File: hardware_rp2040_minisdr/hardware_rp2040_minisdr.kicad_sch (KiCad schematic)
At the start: 0 parts

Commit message: started with schematic
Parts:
- added C1: C, symbol Device:C
- added C10, C11, C12, C13, C14, C15, C6, C7, C9: 100n, symbol Device:C
- added C16, C8: 1u, symbol Device:C
- added C2, C3: 15p, symbol Device:C
- added C4, C5: 10u, symbol Device:C
- added D1: ESDS314DBVR, SOT95P280X145-5N, symbol USER:ESDS314DBVR
- added J1: Conn_Coaxial_Small, symbol Connector:Conn_Coaxial_Small
- added J2: USB_A, symbol Connector:USB_A
- added R1: R, symbol Device:R
- added R2, R3: 27, symbol Device:R
- added R4: 1k, symbol Device:R
- added U1: RP2040, Package_DFN_QFN:QFN-56-1EP_7x7mm_P0.4mm_EP3.2x3.2mm, symbol MCU_RaspberryPi:RP2040
- added U2: W25Q128JVS, Package_SO:SOIC-8_5.3x5.3mm_P1.27mm, symbol Memory_Flash:W25Q128JVS
- added U3: AMS1117-3.3, Package_TO_SOT_SMD:SOT-223-3_TabPin2, symbol Regulator_Linear:AMS1117-3.3
- added Y1: Crystal_GND24, symbol Device:Crystal_GND24
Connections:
- new net: C2.1, R4.1, Y1.1
- new net: R4.2, U1.21 (XOUT)
- new net: C3.2, U1.20 (XIN), Y1.3
- new net: R3.2, U1.46 (USB_DM)
- new net: R2.1, U1.47 (USB_DP)
- new net: C4.1, J2.1 (VBUS), U3.3 (VI)
- new net 1v1: C6.1, C7.1, C8.1, U1.23 (DVDD), U1.45 (VREG_VOUT), U1.50 (DVDD)
- new net 3v3: C10.1, C11.1, C12.1, C13.1, C14.1, C15.1, C16.1, C5.1, C9.1, U1.1 (IOVDD), U1.10 (IOVDD), U1.22 (IOVDD), U1.26 (RUN), U1.33 (IOVDD), U1.42 (IOVDD), U1.43 (ADC_AVDD), U1.44 (VREG_IN), U1.48 (USB_VDD), U1.49 (IOVDD), U2.8 (VCC), U3.2 (VO)
- new net GND: C10.2, C11.2, C12.2, C13.2, C14.2, C15.2, C16.2, C2.2, C3.1, C4.2, C5.2, C6.2, C7.2, C8.2, C9.2, D1.2 (GND), J1.2 (Ext), J2.4 (GND), J2.5 (Shield), U1.19 (TESTEN), U1.57 (GND), U2.4 (GND), U3.1 (GND), Y1.2, Y1.4
- new net QSPI_SCLK: U1.52 (QSPI_SCLK), U2.6 (CLK)
- new net QSPI_SD0: U1.53 (QSPI_SD0), U2.5 (DI/IO_{0})
- new net QSPI_SD1: U1.55 (QSPI_SD1), U2.2 (DO/IO_{1})
- new net QSPI_SD2: U1.54 (QSPI_SD2), U2.3 (~{WP}/IO_{2})
- new net QSPI_SD3: U1.51 (QSPI_SD3), U2.7 (~{HOLD}/~{RESET}/IO_{3})
- new net QSPI_SS: U1.56 (QSPI_SS), U2.1 (~{CS})
- new net SWCLK: U1.24 (SWCLK)
- new net SWD: U1.25 (SWD)
- new net USB_DN: D1.5 (I/O4), J2.2 (D-), R3.1
- new net USB_DP: D1.4 (I/O3), J2.3 (D+), R2.2

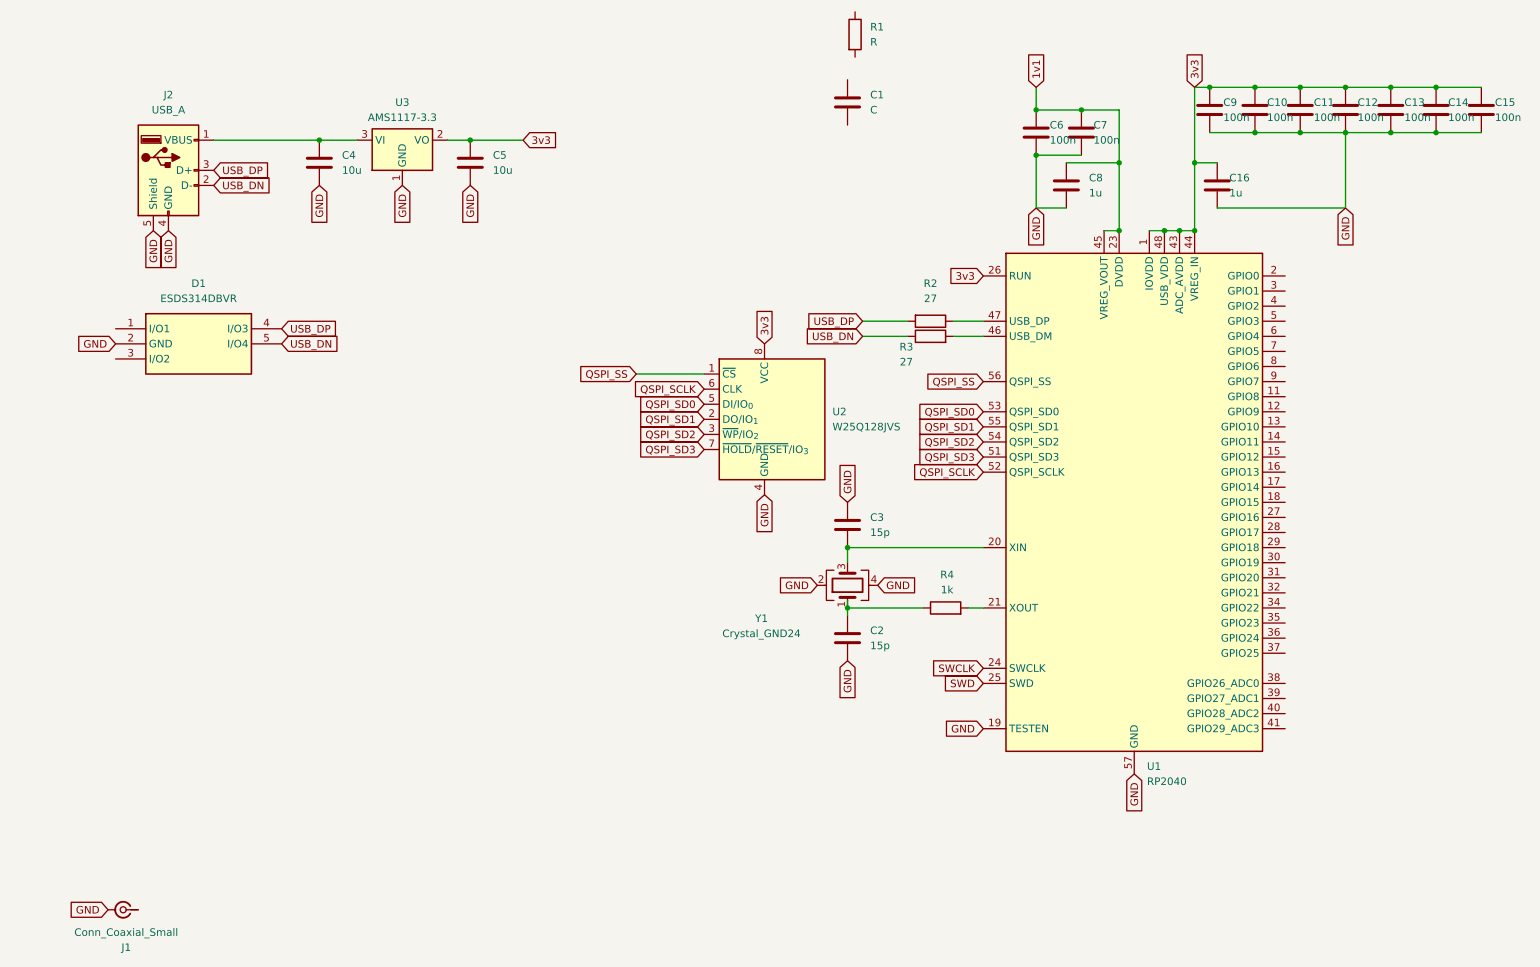
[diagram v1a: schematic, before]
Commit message: schematic
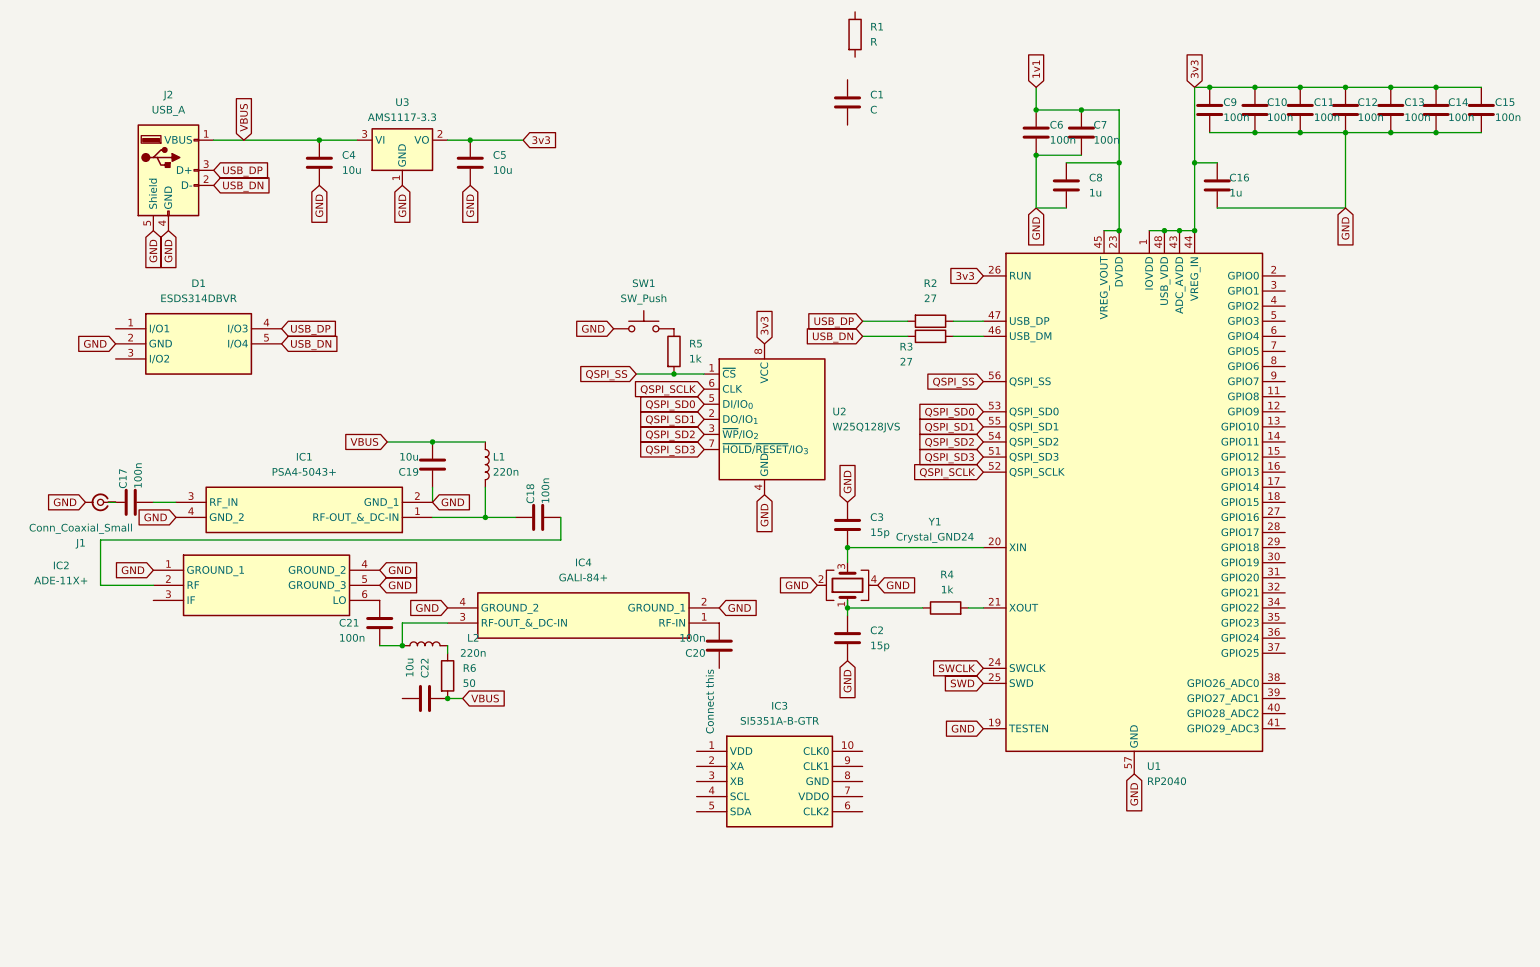
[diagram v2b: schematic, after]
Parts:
- added C17, C18, C20, C21: 100n, symbol Device:C
- added C19, C22: 10u, symbol Device:C
- added IC1: PSA4-5043+, PSA45043, symbol RF:PSA4-5043+
- added IC2: ADE-11X+, SOTFL254P691X284-6N, symbol RF:ADE-11X+
- added IC3: SI5351A-B-GTR, SOP50P490X110-10N, symbol RF:SI5351A-B-GTR
- added IC4: GALI-84+, GALI5, symbol RF:GALI-84+
- added L1, L2: 220n, symbol Device:L
- added R5: 1k, symbol Device:R
- added R6: 50, symbol Device:R
- added SW1: SW_Push, symbol Switch:SW_Push
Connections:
- net GND: now also C19.1, IC1.2 (GND_1), IC1.4 (GND_2), IC2.1 (GROUND_1), IC2.4 (GROUND_2), IC2.5 (GROUND_3), IC4.2 (GROUND_1), IC4.4 (GROUND_2), SW1.1
- net QSPI_SS: now also R5.2
- net at J1.1 (In): now also C17.1
- net VBUS: now reaches C4.1, J2.1 (VBUS), U3.3 (VI)
- net VBUS: now also C19.2, C22.1, L1.1, R6.2
- new net: C21.1, IC2.6 (LO)
- new net: C21.2, IC4.3 (RF-OUT_&_DC-IN), L2.1
- new net: C18.1, IC1.1 (RF-OUT_&_DC-IN), L1.2
- new net: C17.2, IC1.3 (RF_IN)
- new net: C18.2, IC2.2 (RF)
- new net: R5.1, SW1.2
- new net: L2.2, R6.1
- new net: C20.2, IC4.1 (RF-IN)
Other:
- note added: "Connect this"
- moved on the sheet: J1

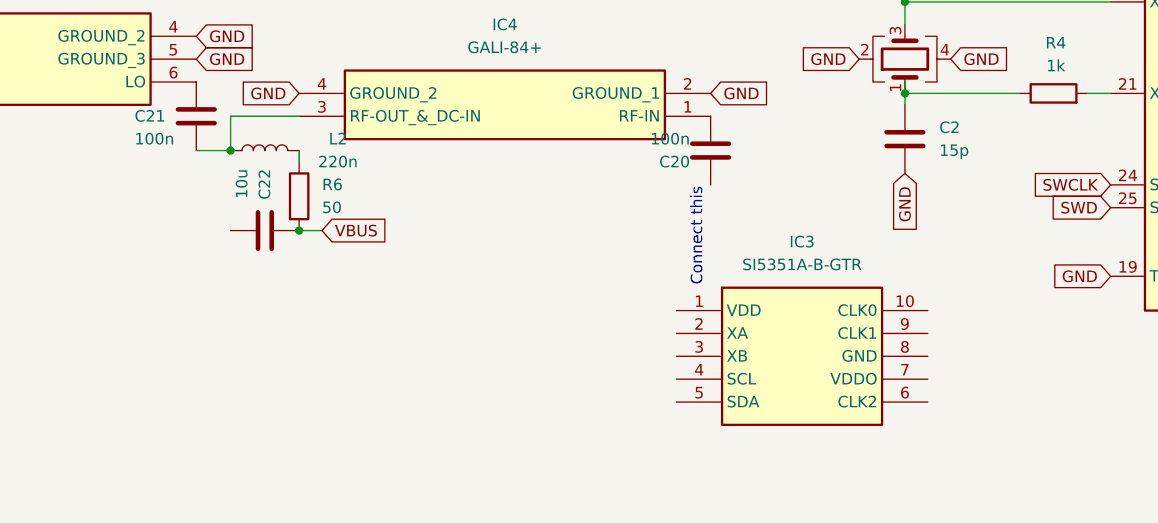
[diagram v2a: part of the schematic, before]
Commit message: schematic
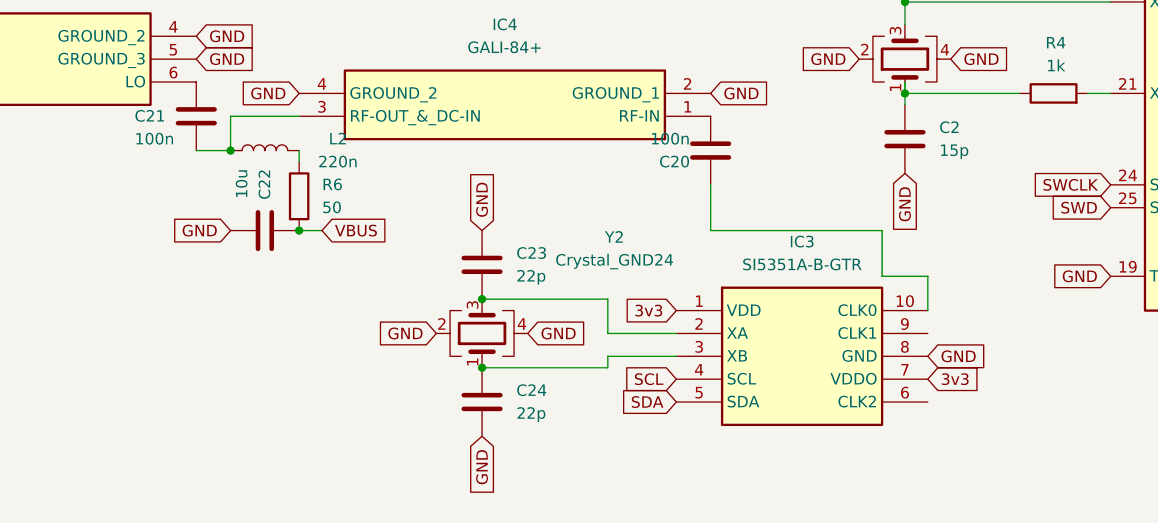
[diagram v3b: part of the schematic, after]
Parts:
- added C23, C24: 22p, symbol Device:C
- added Y2: Crystal_GND24, symbol Device:Crystal_GND24
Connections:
- net 3v3: now also IC3.1 (VDD), IC3.7 (VDDO)
- net GND: now also C22.2, IC3.8 (GND), C23.1, C24.2, Y2.2, Y2.4
- net at IC3.10 (CLK0): now also C20.1
- net at IC3.2 (XA): now also C23.2, Y2.3
- net at IC3.3 (XB): now also C24.1, Y2.1
- net SCL: now reaches IC3.4 (SCL)
- net SDA: now reaches IC3.5 (SDA)
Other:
- note removed: "Connect this"

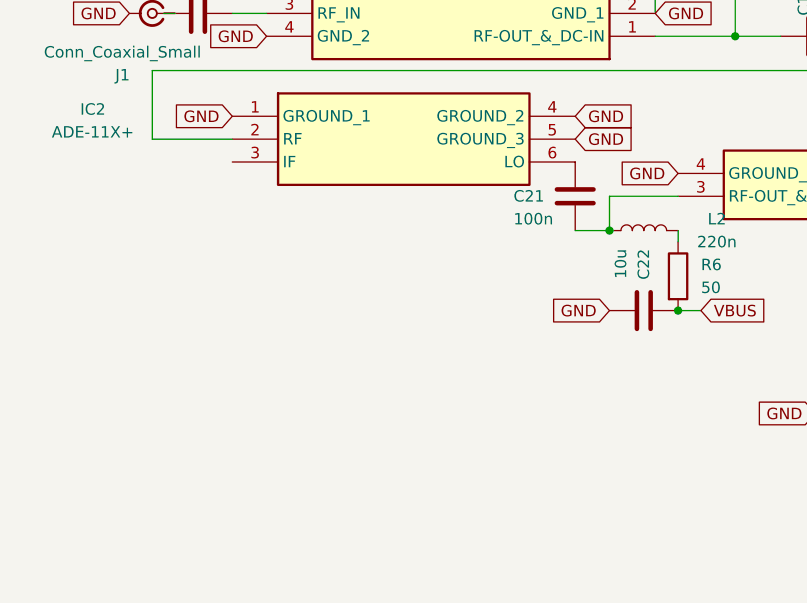
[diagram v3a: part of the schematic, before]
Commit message: schematic
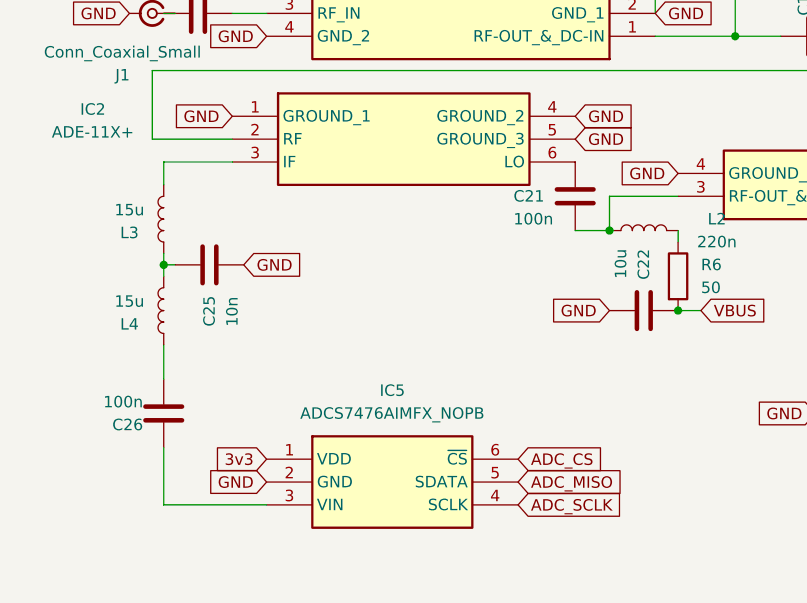
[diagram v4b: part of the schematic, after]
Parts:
- added C25: 10n, symbol Device:C
- added C26: 100n, symbol Device:C
- added IC5: ADCS7476AIMFX_NOPB, SOT95P280X145-6N, symbol Analog_ADC:ADCS7476AIMFX_NOPB
- added L3, L4: 15u, symbol Device:L
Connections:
- net 3v3: now also IC5.1 (VDD)
- net GND: now also C25.2, IC5.2 (GND)
- net at IC2.3 (IF): now also L3.2
- new net: C25.1, L3.1, L4.2
- new net: C26.1, IC5.3 (VIN)
- new net: C26.2, L4.1
- new net ADC_CS: IC5.6 (~{CS})
- new net ADC_MISO: IC5.5 (SDATA)
- new net ADC_SCLK: IC5.4 (SCLK)
